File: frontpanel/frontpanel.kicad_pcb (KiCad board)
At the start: 2 copper layers, 114.9 x 125.5 mm, 1 part

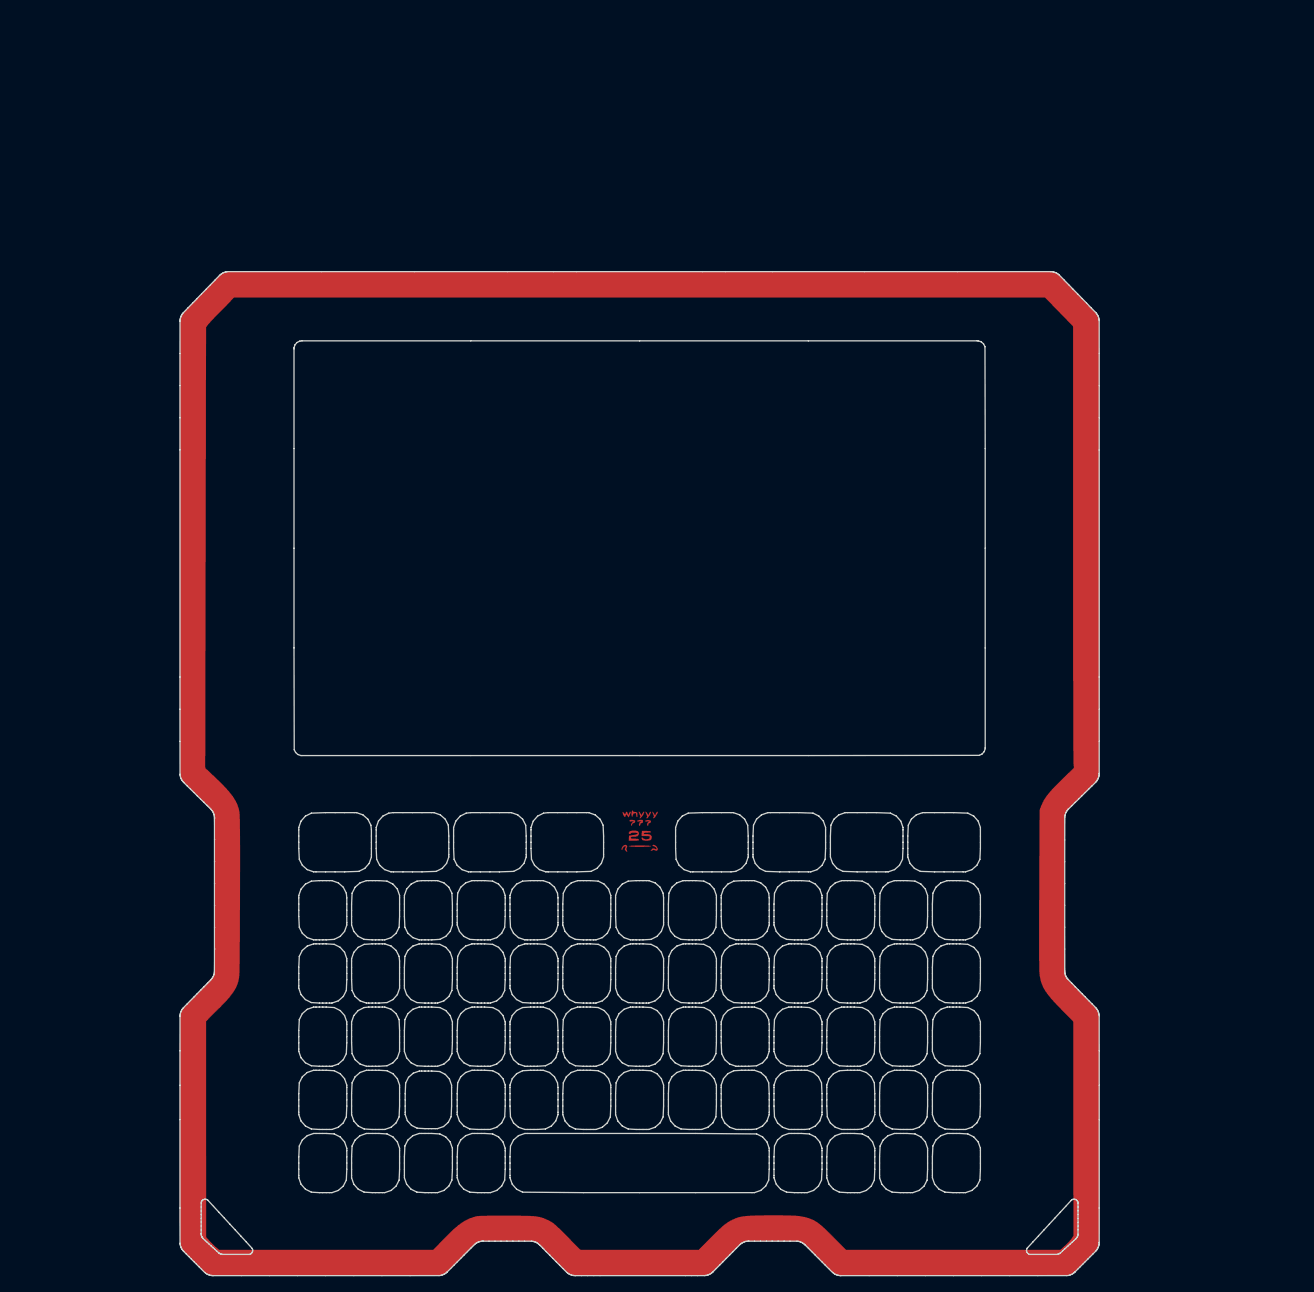
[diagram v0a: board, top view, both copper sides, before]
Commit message: Work in progress
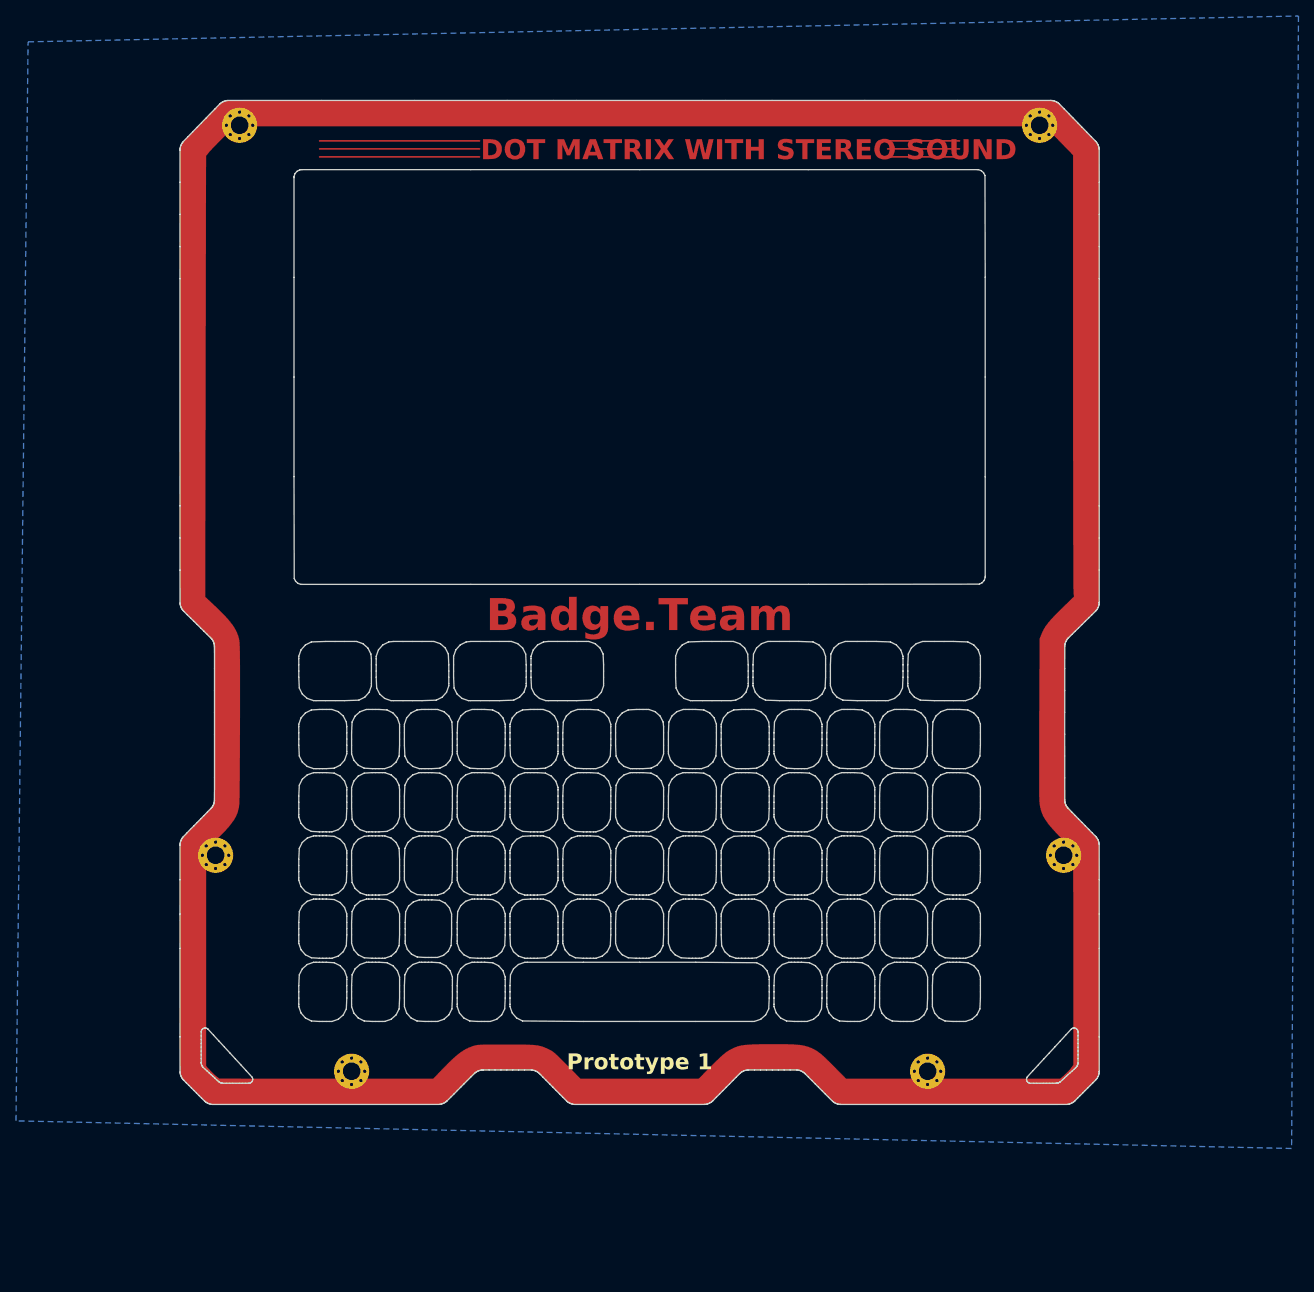
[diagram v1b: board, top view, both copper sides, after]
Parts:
- added H1: ~, MountingHole:MountingHole_2.2mm_M2_Pad_Via, F.Cu at (-50.0, -88.2)
- added H2: ~, MountingHole:MountingHole_2.2mm_M2_Pad_Via, F.Cu at (50.0, -88.2)
- added H3: ~, MountingHole:MountingHole_2.2mm_M2_Pad_Via, F.Cu at (-36.0, 30.0)
- added H4: ~, MountingHole:MountingHole_2.2mm_M2_Pad_Via, F.Cu at (36.0, 30.0)
- added H5: ~, MountingHole:MountingHole_2.2mm_M2_Pad_Via, F.Cu at (-53.0, 3.00)
- added H6: ~, MountingHole:MountingHole_2.2mm_M2_Pad_Via, F.Cu at (53.0, 3.00)
- N1: footprint proto1_kicad_art:proto1_kicad_art -> design:proto1_kicad_art2
- moved N1 21.4 mm to (0.00, -21.4)
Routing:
- added copper zone on B.Cu, net GND
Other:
- board text added: "Badge.Team"
- board text added: "DOT MATRIX WITH STEREO SOUND"
- board text added: "Prototype 1"
